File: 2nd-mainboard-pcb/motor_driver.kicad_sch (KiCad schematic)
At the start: 15 parts, among them J10 Servo Motor BL Touch, J11 T3, J7 Stepper Motor, J8 Servo Motor SM, J9 Microstepping, U11 TMC2209_SILENTSTEPSTICK, U12 MPU-6050

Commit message: cad files gebastelt
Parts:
- A1: footprint Module:Pololu_Breakout-16_15.2x20.3mm -> Imported_Component_Footprints:drv8825
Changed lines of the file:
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@@
 			)
 		)
-		(property "Footprint" "Module:Pololu_Breakout-16_15.2x20.3mm"
+		(property "Footprint" "Imported_Component_Footprints:drv8825"
 			(at 63.5 80.01 0)
 			(effects

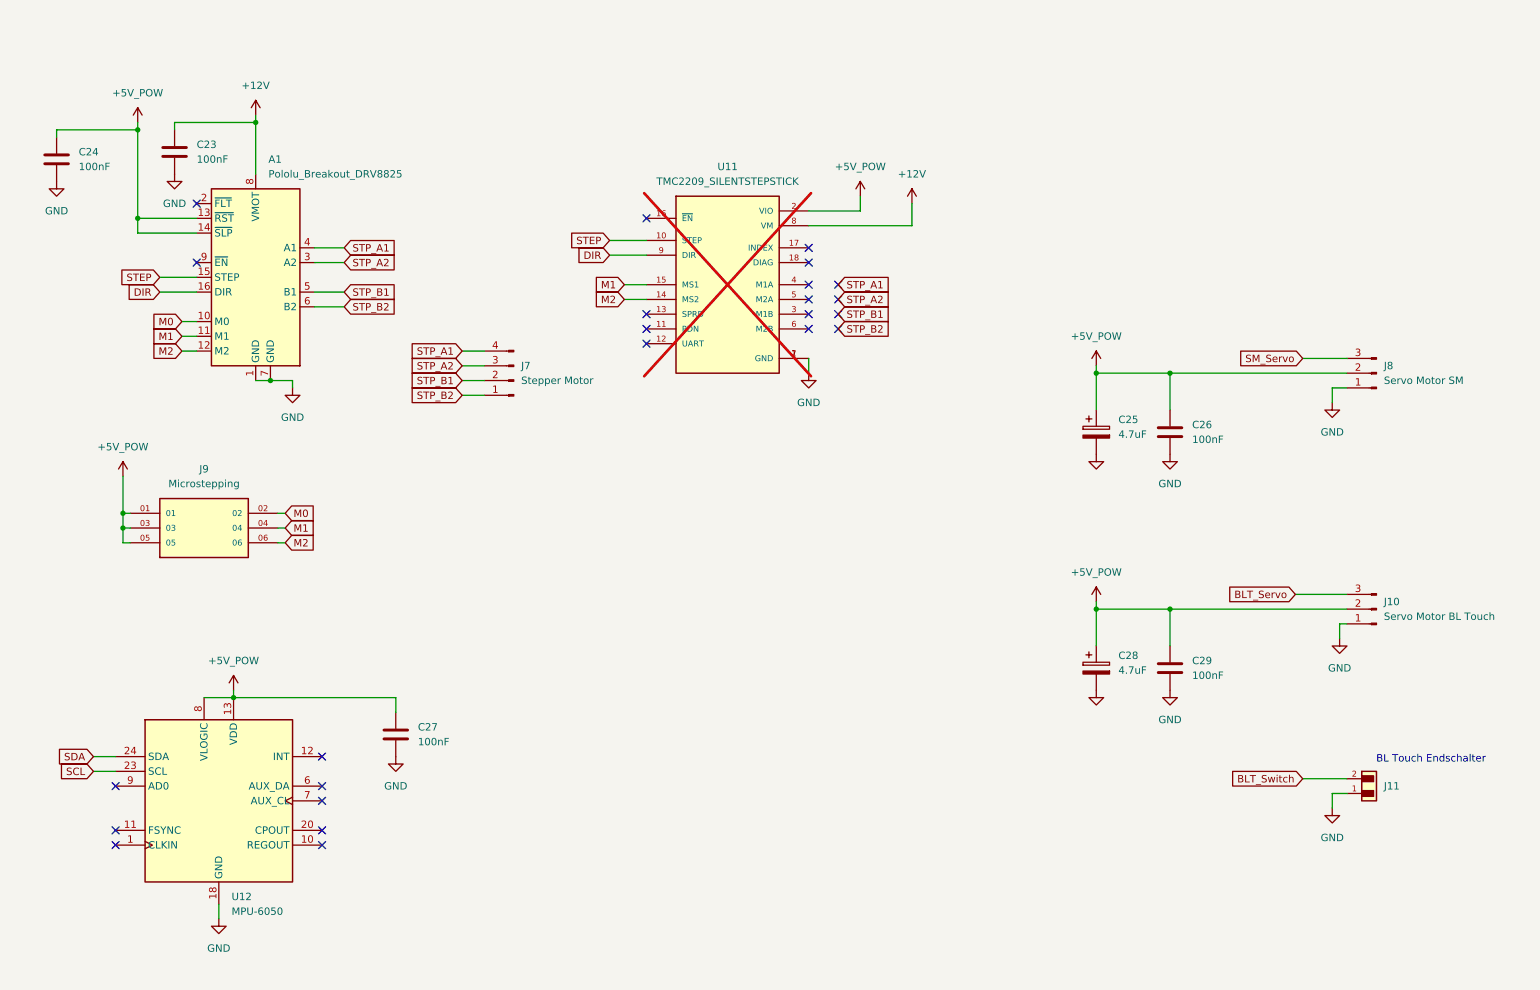
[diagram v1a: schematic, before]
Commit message: stacked pcb reworked
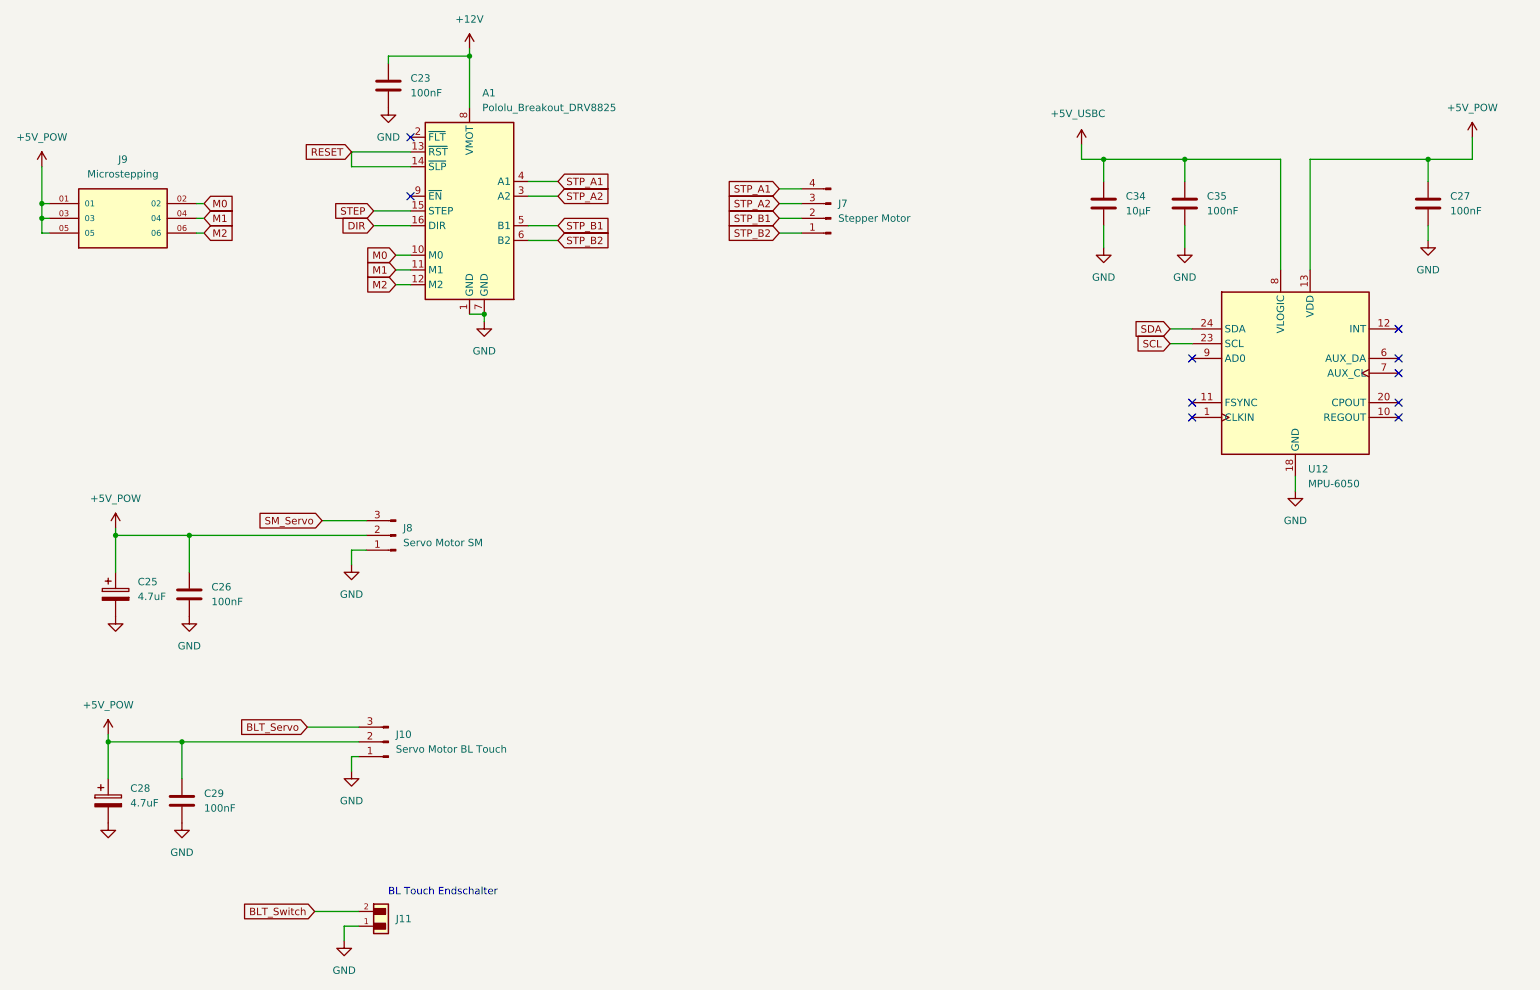
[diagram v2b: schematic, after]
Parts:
- removed C24: 100nF, Capacitor_SMD:C_0402_1005Metric_Pad0.74x0.62mm_HandSolder, symbol Device:C
- removed U11: TMC2209_SILENTSTEPSTICK, Imported_Component_Footprints:MODULE_TMC2209_SILENTSTEPSTICK, symbol Imported_Component_Symbols:TMC2209_SILENTSTEPSTICK
- added C34: 10µF, Capacitor_SMD:C_0805_2012Metric_Pad1.18x1.45mm_HandSolder, symbol Device:C
- added C35: 100nF, Capacitor_SMD:C_0402_1005Metric_Pad0.74x0.62mm_HandSolder, symbol Device:C
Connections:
- net +5V_POW: no longer A1.13 (~{RST}), A1.14 (~{SLP}), U12.8 (VLOGIC)
- net GND: now also C34.2, C35.2
- new net +5V_USBC: C34.1, C35.1, U12.8 (VLOGIC)
- new net RESET: A1.13 (~{RST}), A1.14 (~{SLP})
- no-connect marks 24 -> 10
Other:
- moved on the sheet: A1, C23, C25, C26, C27, C28, C29, J10, J11, J7, J8, J9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

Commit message: rearragned componentens
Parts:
- C23, C26, C27, C29, C35: footprint Capacitor_SMD:C_0402_1005Metric_Pad0.74x0.62mm_HandSolder -> Capacitor_SMD:C_0603_1608Metric_Pad1.08x0.95mm_HandSolder
- C28: footprint Capacitor_SMD:C_0805_2012Metric_Pad1.18x1.45mm_HandSolder -> Capacitor_SMD:C_0603_1608Metric_Pad1.08x0.95mm_HandSolder
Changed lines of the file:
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@@
 			)
 		)
-		(property "Footprint" "Capacitor_SMD:C_0402_1005Metric_Pad0.74x0.62mm_HandSolder"
+		(property "Footprint" "Capacitor_SMD:C_0603_1608Metric_Pad1.08x0.95mm_HandSolder"
 			(at 261.3152 53.34 0)
 			(effects
@@
 			)
 		)
-		(property "Footprint" "Capacitor_SMD:C_0402_1005Metric_Pad0.74x0.62mm_HandSolder"
+		(property "Footprint" "Capacitor_SMD:C_0603_1608Metric_Pad1.08x0.95mm_HandSolder"
 			(at 219.4052 53.34 0)
 			(effects
@@
 			)
 		)
-		(property "Footprint" "Capacitor_SMD:C_0402_1005Metric_Pad0.74x0.62mm_HandSolder"
+		(property "Footprint" "Capacitor_SMD:C_0603_1608Metric_Pad1.08x0.95mm_HandSolder"
 			(at 46.6852 156.21 0)
 			(effects
@@
 			)
 		)
-		(property "Footprint" "Capacitor_SMD:C_0805_2012Metric_Pad1.18x1.45mm_HandSolder"
+		(property "Footprint" "Capacitor_SMD:C_0603_1608Metric_Pad1.08x0.95mm_HandSolder"
 			(at 33.9852 156.21 0)
 			(effects
@@
 			)
 		)
-		(property "Footprint" "Capacitor_SMD:C_0402_1005Metric_Pad0.74x0.62mm_HandSolder"
+		(property "Footprint" "Capacitor_SMD:C_0603_1608Metric_Pad1.08x0.95mm_HandSolder"
 			(at 82.2452 33.02 0)
 			(effects
@@
 			)
 		)
-		(property "Footprint" "Capacitor_SMD:C_0402_1005Metric_Pad0.74x0.62mm_HandSolder"
+		(property "Footprint" "Capacitor_SMD:C_0603_1608Metric_Pad1.08x0.95mm_HandSolder"
 			(at 47.9552 120.65 0)
 			(effects
